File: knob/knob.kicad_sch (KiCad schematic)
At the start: 10 parts, among them SW1 SW_Push, SW2 SW_Push, SW3 SW_Push, SW4 SW_Push, SW5 SW_Push, SW6 SW_Push, SW7 RotaryEncoder_Switch, SW8 RotaryEncoder_Switch

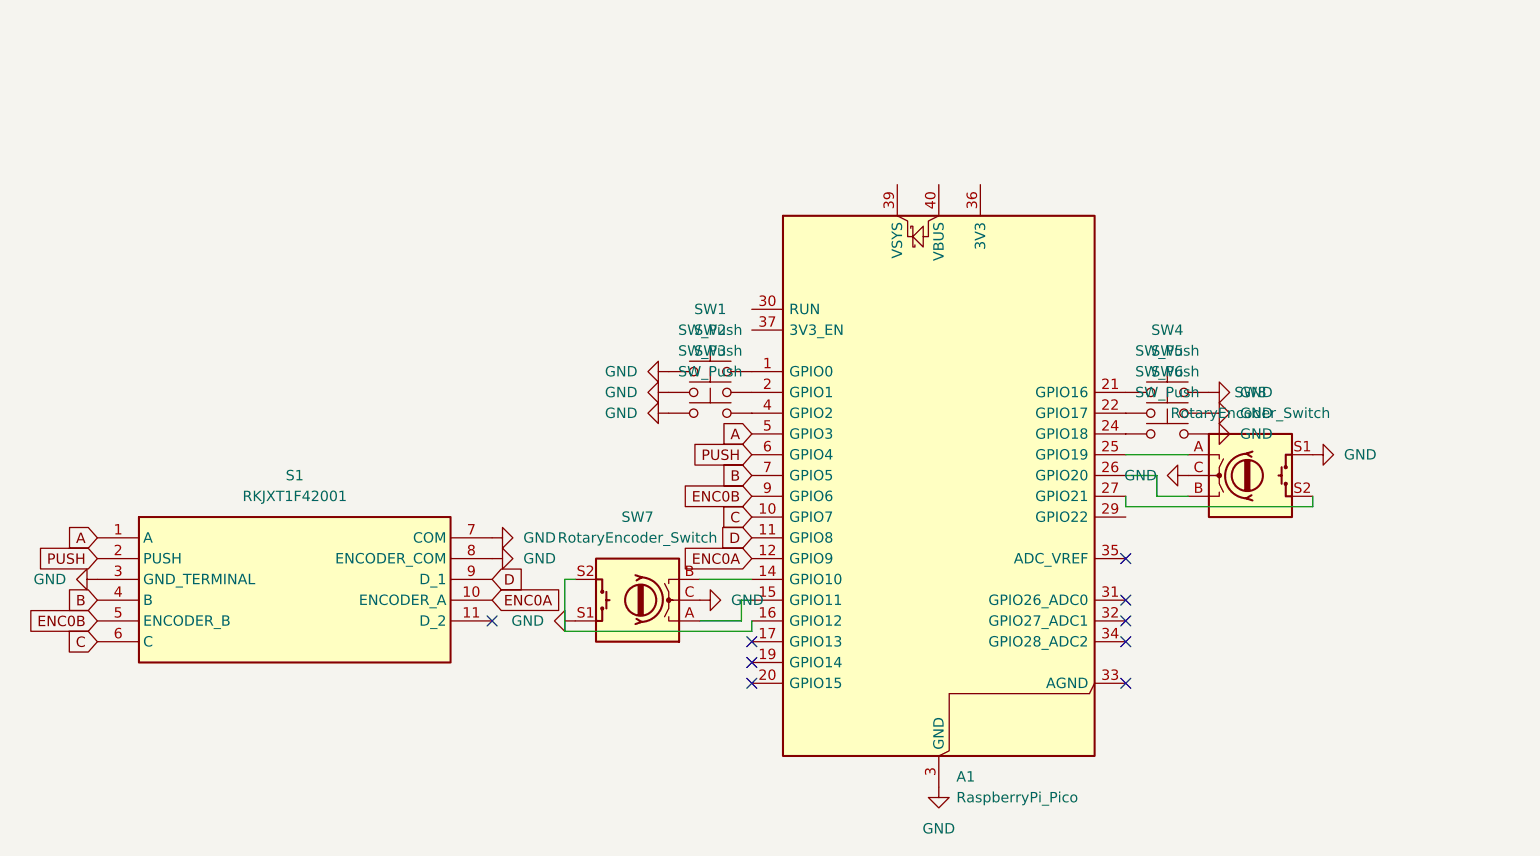
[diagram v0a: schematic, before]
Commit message: sync
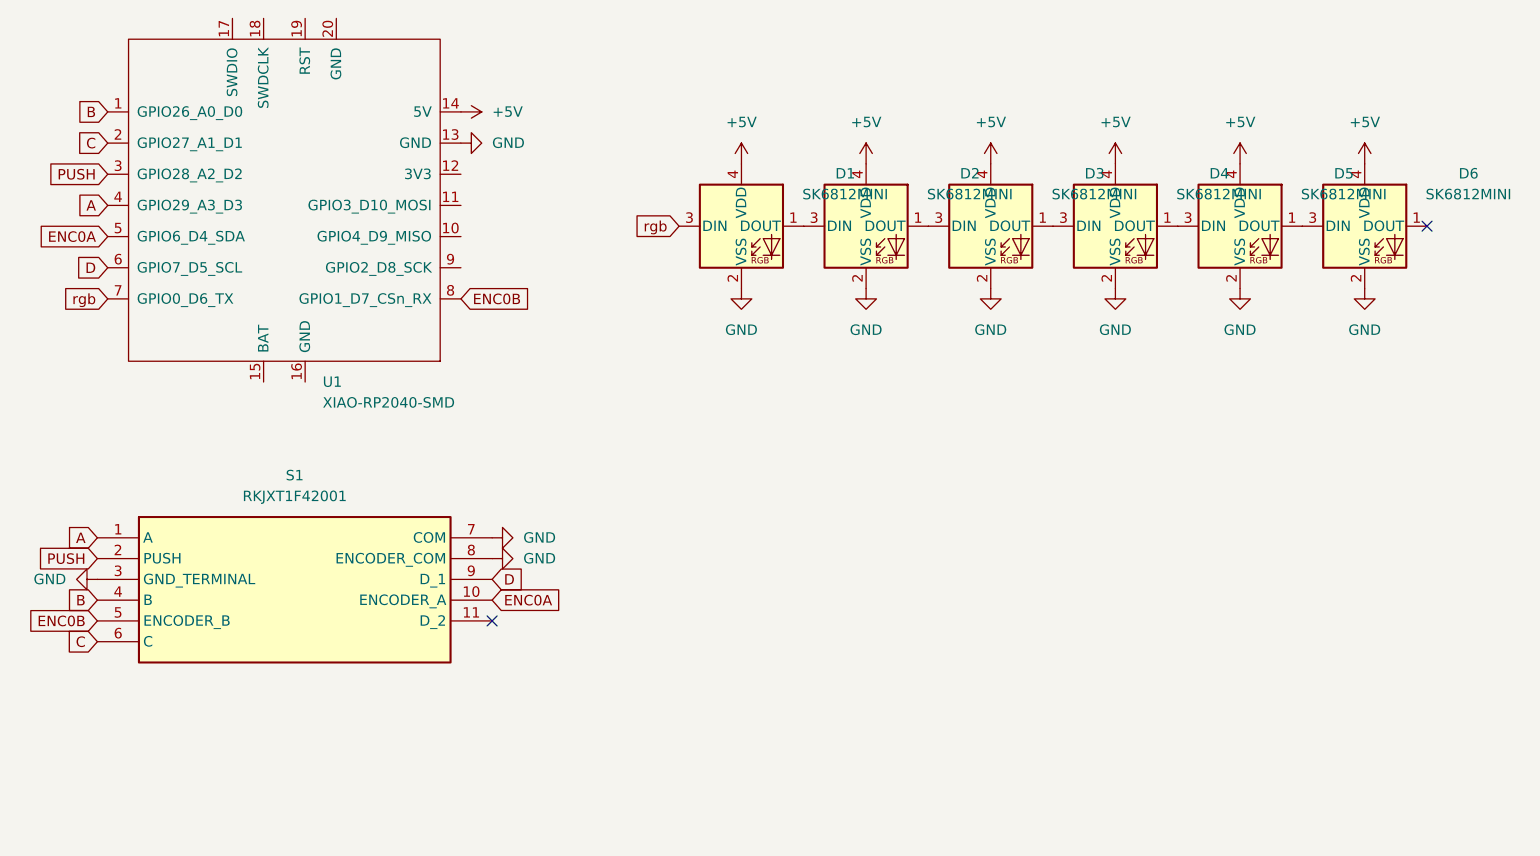
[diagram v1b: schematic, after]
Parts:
- removed A1: RaspberryPi_Pico, Module:RaspberryPi_Pico_Common_Unspecified, symbol MCU_Module:RaspberryPi_Pico
- removed SW1, SW2, SW3, SW4, SW5, SW6: SW_Push, Button_Switch_Keyboard:SW_Cherry_MX_1.00u_PCB, symbol Switch:SW_Push
- removed SW7, SW8: RotaryEncoder_Switch, Rotary_Encoder:RotaryEncoder_Alps_EC11E-Switch_Vertical_H20mm_MountingHoles, symbol Device:RotaryEncoder_Switch
- added D1, D2, D3, D4, D5, D6: SK6812MINI, cheyao macropad main PCB-third_party_neopixel.petty:SK6812MINI-E, symbol LED:SK6812MINI
- added U1: XIAO-RP2040-SMD, Seeed Studio XIAO Series Library:XIAO-RP2040-SMD, symbol Seeed_Studio_XIAO_Series:XIAO-RP2040-SMD
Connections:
- net A: now also U1.4 (GPIO29_A3_D3)
- net B: now also U1.1 (GPIO26_A0_D0)
- net C: now also U1.2 (GPIO27_A1_D1)
- net D: now also U1.6 (GPIO7_D5_SCL)
- net ENC0A: now also U1.5 (GPIO6_D4_SDA)
- net ENC0B: now also U1.8 (GPIO1_D7_CSn_RX)
- net GND: now also D1.2 (VSS), D2.2 (VSS), D3.2 (VSS), D4.2 (VSS), D5.2 (VSS), D6.2 (VSS), U1.13 (GND)
- net PUSH: now also U1.3 (GPIO28_A2_D2)
- new net: D4.1 (DOUT), D5.3 (DIN)
- new net: D3.1 (DOUT), D4.3 (DIN)
- new net: D2.1 (DOUT), D3.3 (DIN)
- new net: D1.1 (DOUT), D2.3 (DIN)
- new net: D5.1 (DOUT), D6.3 (DIN)
- new net +5V: D1.4 (VDD), D2.4 (VDD), D3.4 (VDD), D4.4 (VDD), D5.4 (VDD), D6.4 (VDD), U1.14 (5V)
- new net rgb: D1.3 (DIN), U1.7 (GPIO0_D6_TX)
- no-connect marks 9 -> 2
